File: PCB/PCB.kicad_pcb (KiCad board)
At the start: 6 copper layers, 22 x 80 mm, 270 parts, among them J1 Bus_M.2_Edge_M, J2 Conn_ARM_SWD_TagConnect_TC2030, J4 TYPE-C-31-M-12, J7 HDMI_D_1.4, SW1 SW_Push, U1 XC7A50T-FGG484, U10 FT2232HQ, U11 MT41J128M16JT-125:K, U12 PCA9306DC1, U14 UCL0524P, U15 UCL0524P, U16 UCL0524P, U17 TPS62132, U2 MAX20029ATIA/V+, U3 TPD2EUSB30, U4 TPD2EUSB30, U5 TPS2121RUXR, U6 TPD2EUSB30, U7 MT25QL128ABA1EW7-0SIT, U9 M93C56-WMN6TP, Y2 12MHz, Y3 100MHz

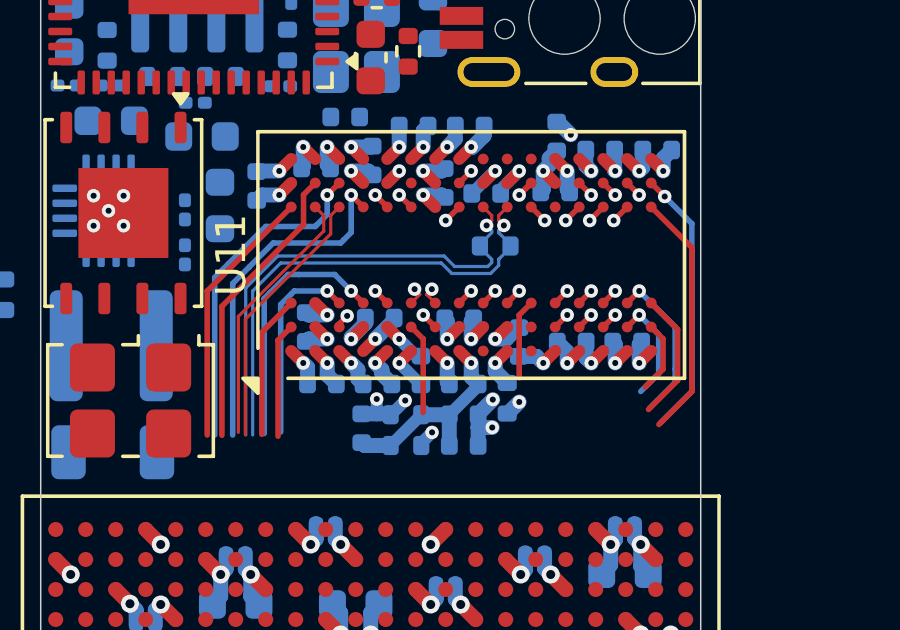
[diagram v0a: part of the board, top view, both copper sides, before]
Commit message: finished the IO fanout
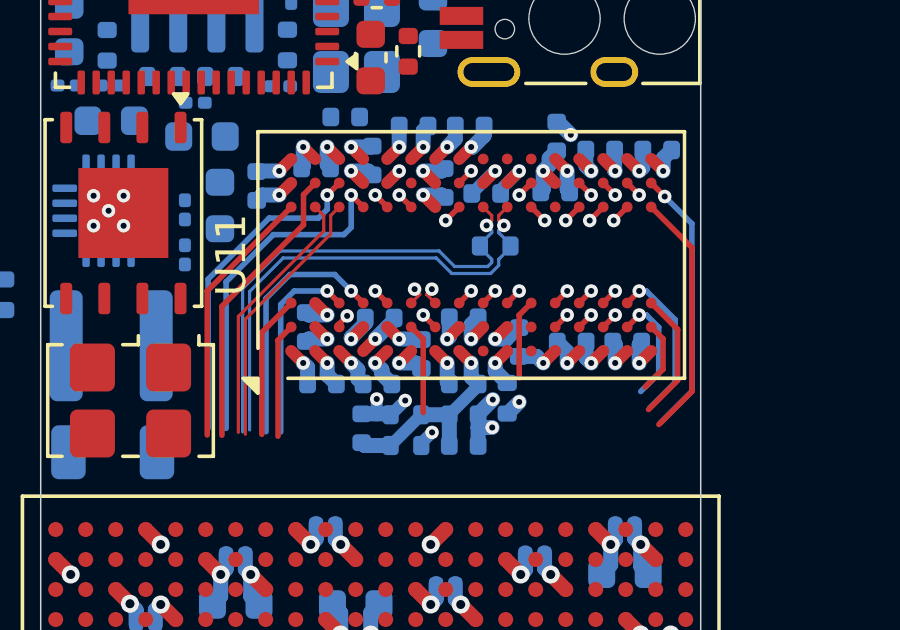
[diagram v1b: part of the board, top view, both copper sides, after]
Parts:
- moved C82 0.55 mm to (145.4, 81.2)
- moved C63 0.15 mm to (146.8, 79.9)
